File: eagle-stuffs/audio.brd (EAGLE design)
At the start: 57.1 x 44.5 mm, 27 parts, among them IC2 TL084P, IC3 DS1804, IC4 DS1804, U1 AT42QT1010SOT23, U2 SSM2211SZ

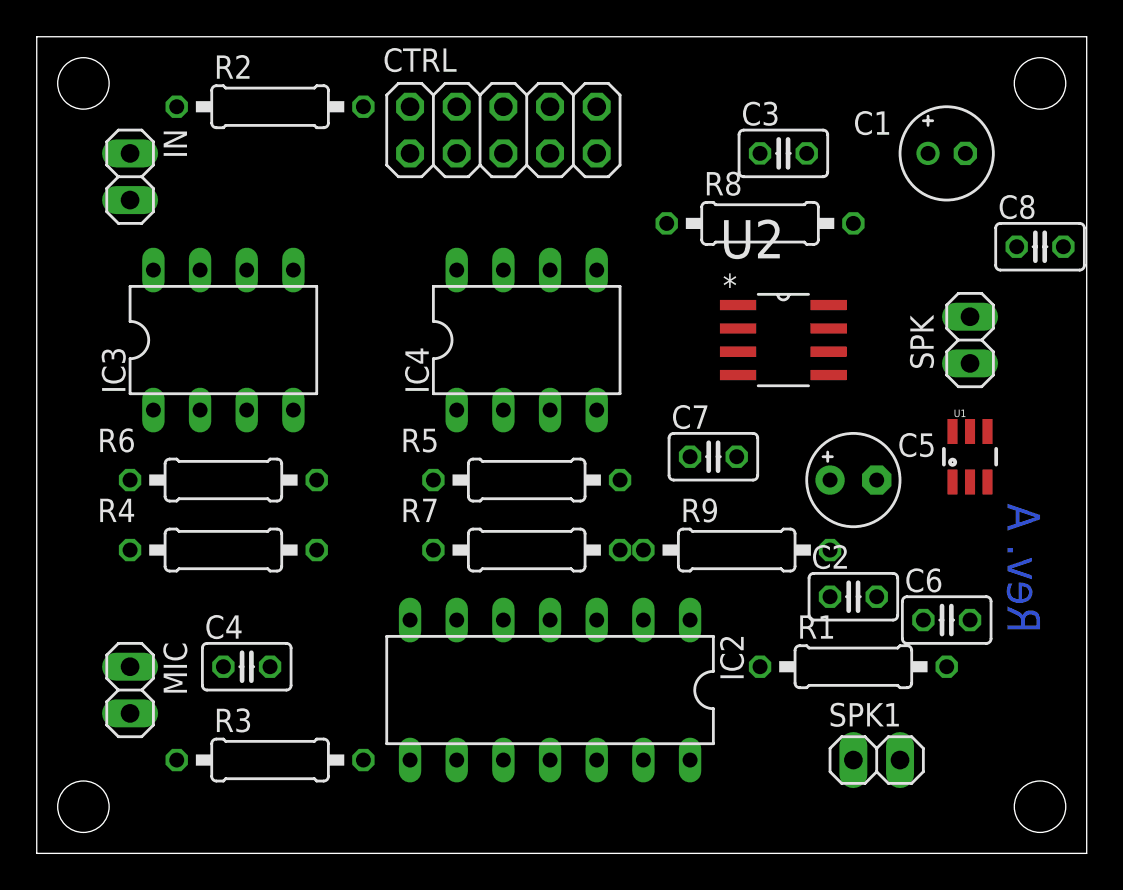
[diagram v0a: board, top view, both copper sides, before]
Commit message: This should work…
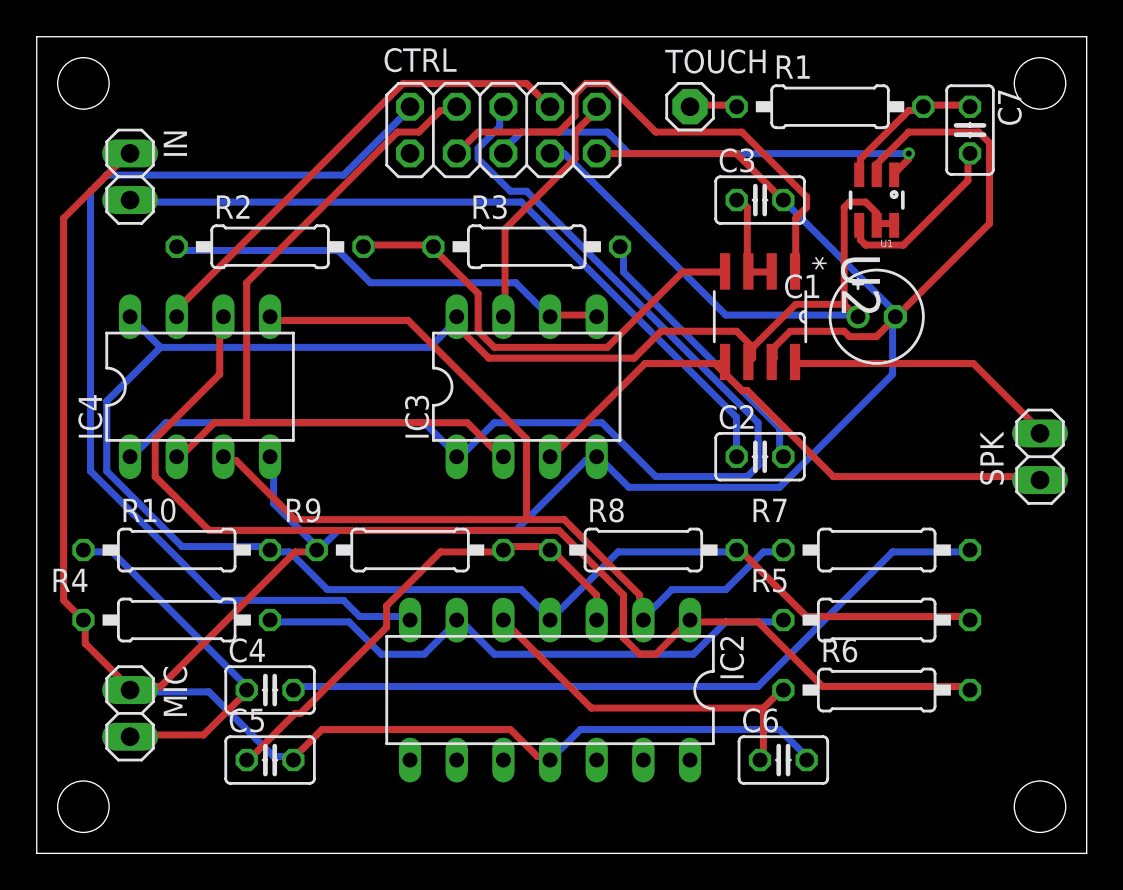
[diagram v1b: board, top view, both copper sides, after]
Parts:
- removed C8: 2.2nF, rcl:C025-025X050
- removed SPK1: (no value), pinhead:1X02
- added R10: 10K, resistor:0207/10
- added TOUCH: (no value), adafruit:1X01
- C2: value 0.01u -> 2.2
- C3: value 0.047u -> 2.2
- C5: value 100uF -> 1; device rcl:E2,5-5 -> rcl:C025-025X050
- C6: value 10nF -> 2.2nF
- C7: value 1 -> 10nF
- IC3: value DS1804 -> DS1804-10k
- R2: value 10 -> 8k
- R3: value 10K -> 10k
- R4: value 100K -> 15K
- R6: value 15K -> 33K
- R9: value 33K -> 100K
- moved R6 37.4 mm to (45.7, 8.89)
- moved C5 35.2 mm to (12.7, 5.08)
- moved R3 31.2 mm to (26.7, 33.0)
- moved R1 30.5 mm to (43.2, 40.6)
- moved C7 22.6 mm to (50.8, 39.4), turned to 270 degrees
- moved R5 20.5 mm to (45.7, 12.7)
- moved R7 19.0 mm to (45.7, 16.5)
- moved R8 18.9 mm to (33.0, 16.5)
- moved IC4 18.0 mm to (8.89, 25.4)
- moved R9 17.8 mm to (20.3, 16.5)
- moved IC3 16.7 mm to (26.7, 25.4)
- moved U1 14.9 mm to (45.7, 35.6), turned to 180 degrees
- moved C6 11.7 mm to (40.6, 5.08)
- moved C1 9.67 mm to (45.7, 29.2)
- moved C2 9.16 mm to (39.4, 21.6)
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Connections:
- removed net V+: U2.6
- removed net V-: U2.7
- new net N$2: C2.1, IN.2
- new net N$3: C2.2, R3.2
- new net N$4: R2.2, R3.1, U2.4
- new net N$5: C3.1, U2.2, U2.3
- new net N$6: SPK.1, U2.8
- new net N$7: IC3.5, IC3.6, R2.1
- net +5V: now also C1.+, IC3.8, R10.2, U2.6; no longer R3.2
- net GND: now also C1.-, C3.2, C5.2, C6.2, R9.1, U2.7; no longer C7.2, C8.2, R6.1, SPK.2
- net N$1: now also IC3.3, SPK.2, U2.5; no longer IC3.5
- net N$11: now also R6.2; no longer R9.2
- net N$12: now also R4.2; no longer R6.2
- net N$13: now also C6.1, R6.1; no longer C8.1, R9.1
- net N$15: now also C5.1, R9.2; no longer C7.1, R4.2
- net N$16: now also C7.1; no longer C6.1
- net N$17: now also C7.2; no longer C6.2
- net N$22: now also TOUCH.1; no longer SPK1.1
- net N$9: now also R10.1; no longer R3.1
- net VCC: now also CTRL.8, U2.1; no longer IC3.8
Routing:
- net GND: track 0.00 -> 180.9 mm
- net +5V: track 0.00 -> 137.4 mm
- net N$20: track 0.00 -> 64.9 mm
- net N$11: track 0.00 -> 62.3 mm
- net N$10: track 0.00 -> 57.6 mm
- net N$14: track 0.00 -> 55.4 mm
- net N$21: track 0.00 -> 42.4 mm
- net N$2: track 0.00 -> 40.0 mm
- net N$8: track 0.00 -> 40.0 mm
- net N$1: track 0.00 -> 32.0 mm
- net N$12: track 0.00 -> 31.0 mm
- net VCC: track 0.00 -> 28.2 mm
- net N$15: track 0.00 -> 27.0 mm
- net N$19: track 0.00 -> 26.4 mm
- net N$4: track 0.00 -> 25.0 mm
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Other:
- board text removed: "Rev. A"

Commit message: Waiting for proto board test design
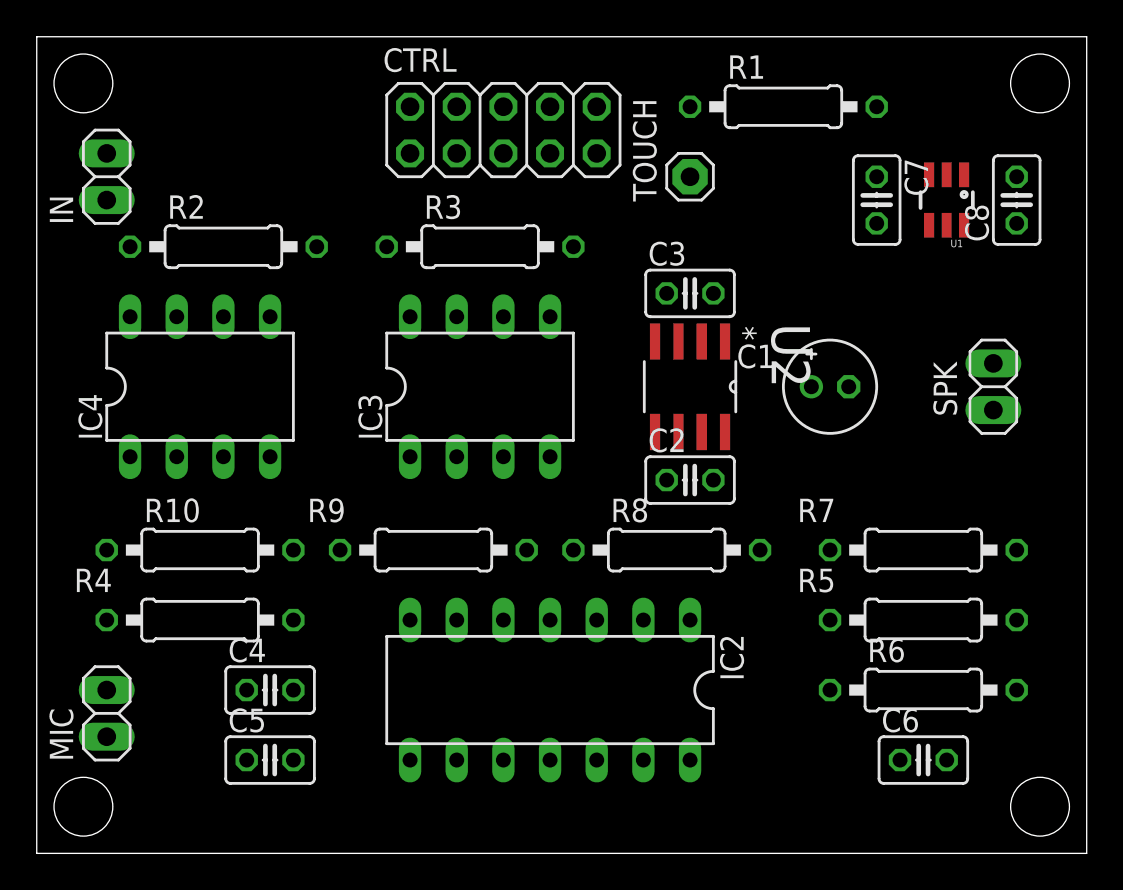
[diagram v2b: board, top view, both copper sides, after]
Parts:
- added C8: 0.1, rcl:C025-025X050
- C4: value 0.1 -> 1
- C7: value 10nF -> 0.01
- R10: value 10K -> 1k
- moved C6 7.62 mm to (48.3, 5.08)
- moved C3 6.35 mm to (35.6, 30.5)
- moved C7 6.35 mm to (45.7, 35.6)
- moved U2 5.39 mm to (35.6, 25.4)
- moved C1 4.58 mm to (43.2, 25.4)
- moved SPK 4.58 mm to (52.1, 25.4)
- moved C2 4.02 mm to (35.6, 20.3)
- moved TOUCH 3.81 mm to (35.6, 36.8), turned to 90 degrees
- moved U1 3.81 mm to (49.5, 35.6)
- moved IC3 2.54 mm to (24.1, 25.4)
- moved R3 2.54 mm to (24.1, 33.0)
- moved R1 2.54 mm to (40.6, 40.6)
- moved R2 2.54 mm to (10.2, 33.0)
- moved R5 2.54 mm to (48.3, 12.7)
- moved R6 2.54 mm to (48.3, 8.89)
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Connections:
- net +5V: now also C8.1
- net GND: now also C8.2
- net N$10: no longer IC4.3
- net N$7: no longer IC3.6
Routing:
- net GND: track 180.9 -> 0.00 mm
- net +5V: track 137.4 -> 0.00 mm
- net N$20: track 64.9 -> 0.00 mm
- net N$11: track 62.3 -> 0.00 mm
- net N$10: track 57.6 -> 0.00 mm
- net N$14: track 55.4 -> 0.00 mm
- net N$21: track 42.4 -> 0.00 mm
- net N$2: track 40.0 -> 0.00 mm
- net N$8: track 40.0 -> 0.00 mm
- net N$1: track 32.0 -> 0.00 mm
- net N$12: track 31.0 -> 0.00 mm
- net VCC: track 28.2 -> 0.00 mm
- net N$15: track 27.0 -> 0.00 mm
- net N$19: track 26.4 -> 0.00 mm
- net N$4: track 25.0 -> 0.00 mm
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
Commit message: Final beta
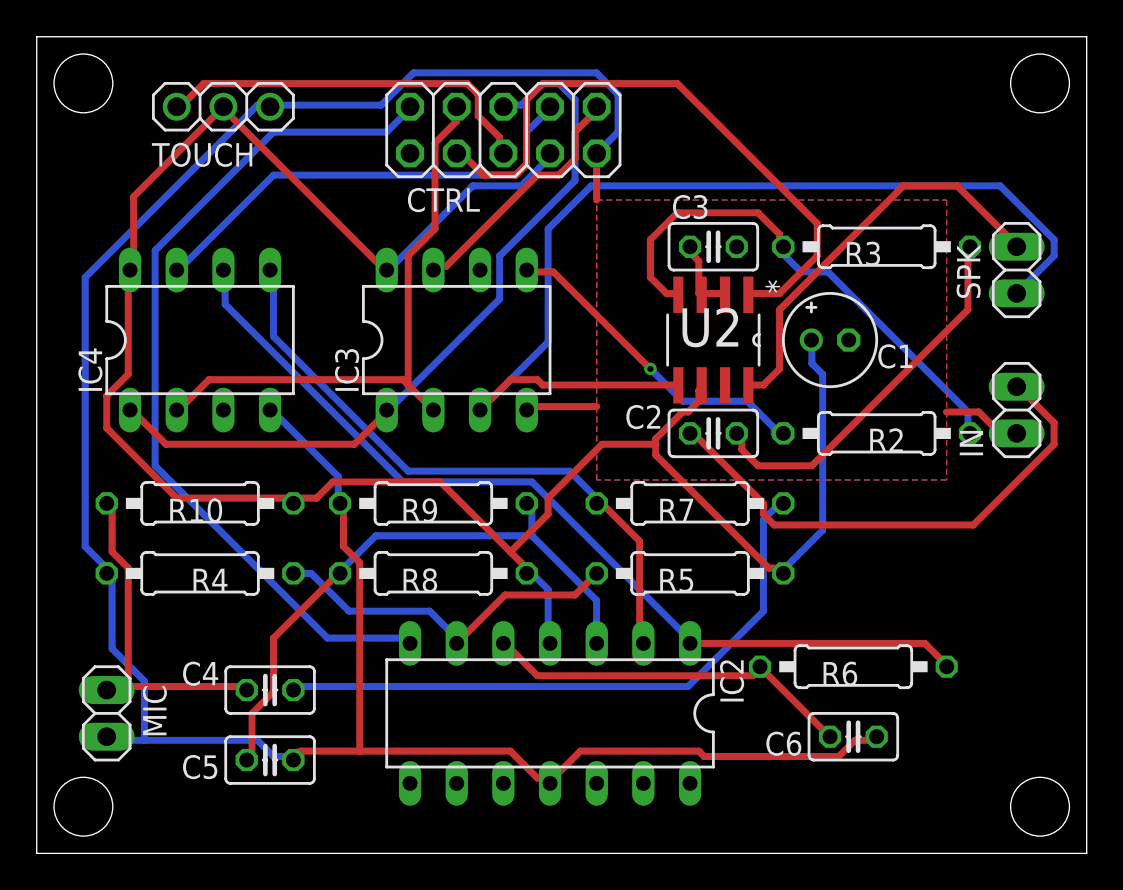
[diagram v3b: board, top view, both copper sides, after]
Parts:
- removed C7: 0.01, rcl:C025-025X050
- removed C8: 0.1, rcl:C025-025X050
- removed R1: 10k, resistor:0207/10
- removed U1: AT42QT1010SOT23, SparkFun-DigitalIC:SOT23-6
- R4: value 15K -> 15k
- R5: value 10K -> 10k
- R6: value 33K -> 33k
- R7: value 1K -> 1k
- R8, R9: value 100K -> 100k
- TOUCH: device adafruit:1X01 -> adafruit:1X03
- moved IN 51.1 mm to (53.3, 24.1)
- moved R2 37.0 mm to (45.7, 22.9)
- moved TOUCH 25.7 mm to (10.2, 40.6), turned to 0 degrees
- moved R3 21.6 mm to (45.7, 33.0)
- moved R5 13.0 mm to (35.6, 15.2)
- moved R7 13.0 mm to (35.6, 19.1)
- moved R8 12.8 mm to (21.6, 15.2)
- moved SPK 6.48 mm to (53.3, 31.8)
- moved C6 4.02 mm to (44.5, 6.35)
- moved R6 4.02 mm to (44.5, 10.2)
- moved IC3 2.84 mm to (22.9, 27.9)
- moved C3 2.84 mm to (36.8, 33.0)
- moved U2 2.84 mm to (36.8, 27.9)
- moved C2 2.84 mm to (36.8, 22.9)
- moved C1 2.54 mm to (43.2, 27.9)
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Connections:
- removed net N$16: C7.1, R1.2, U1.3
- removed net N$17: C7.2, U1.4
- removed net N$24: CTRL.6, U1.1
- net +5V: now also TOUCH.2; no longer C8.1, U1.5, U1.6
- net GND: now also TOUCH.3; no longer C8.2, U1.2
- net N$22: now also CTRL.6; no longer R1.1
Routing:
- net GND: track 0.00 -> 141.0 mm
- net +5V: track 0.00 -> 115.9 mm
- net N$1: track 0.00 -> 56.5 mm
- net N$11: track 0.00 -> 49.5 mm
- net N$14: track 0.00 -> 46.8 mm
- net N$20: track 0.00 -> 41.5 mm
- net N$10: track 0.00 -> 34.1 mm
- net N$8: track 0.00 -> 33.8 mm
- net VCC: track 0.00 -> 33.8 mm
- net N$15: track 0.00 -> 33.0 mm
- net N$21: track 0.00 -> 31.6 mm
- net N$4: track 0.00 -> 28.3 mm
- net N$2: track 0.00 -> 28.0 mm
- net N$19: track 0.00 -> 25.1 mm
- net N$6: track 0.00 -> 22.4 mm
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- added copper zone on layer 1, net GND
- added copper zone on layer 16, net N$16
